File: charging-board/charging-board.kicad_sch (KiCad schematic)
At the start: 53 parts, among them J1 Conn_02x13_Counter_Clockwise, J12 everything_connector, J13 FTSH-107-01-F-DV-K-P-TR, J2 Conn_01x04, J6 TSMP_to_HV, J7 TSMP_to_Banana Jacks, J8 J1772_Negotiation, SW1 Y97KT23B5NAFP, U1 AP63205WU, U2 ISO1044BD, U3 STM32G441KBTx, U7 MIC5504-3.3YM5, Y2 ECS-240-8-37B-CKY-TR

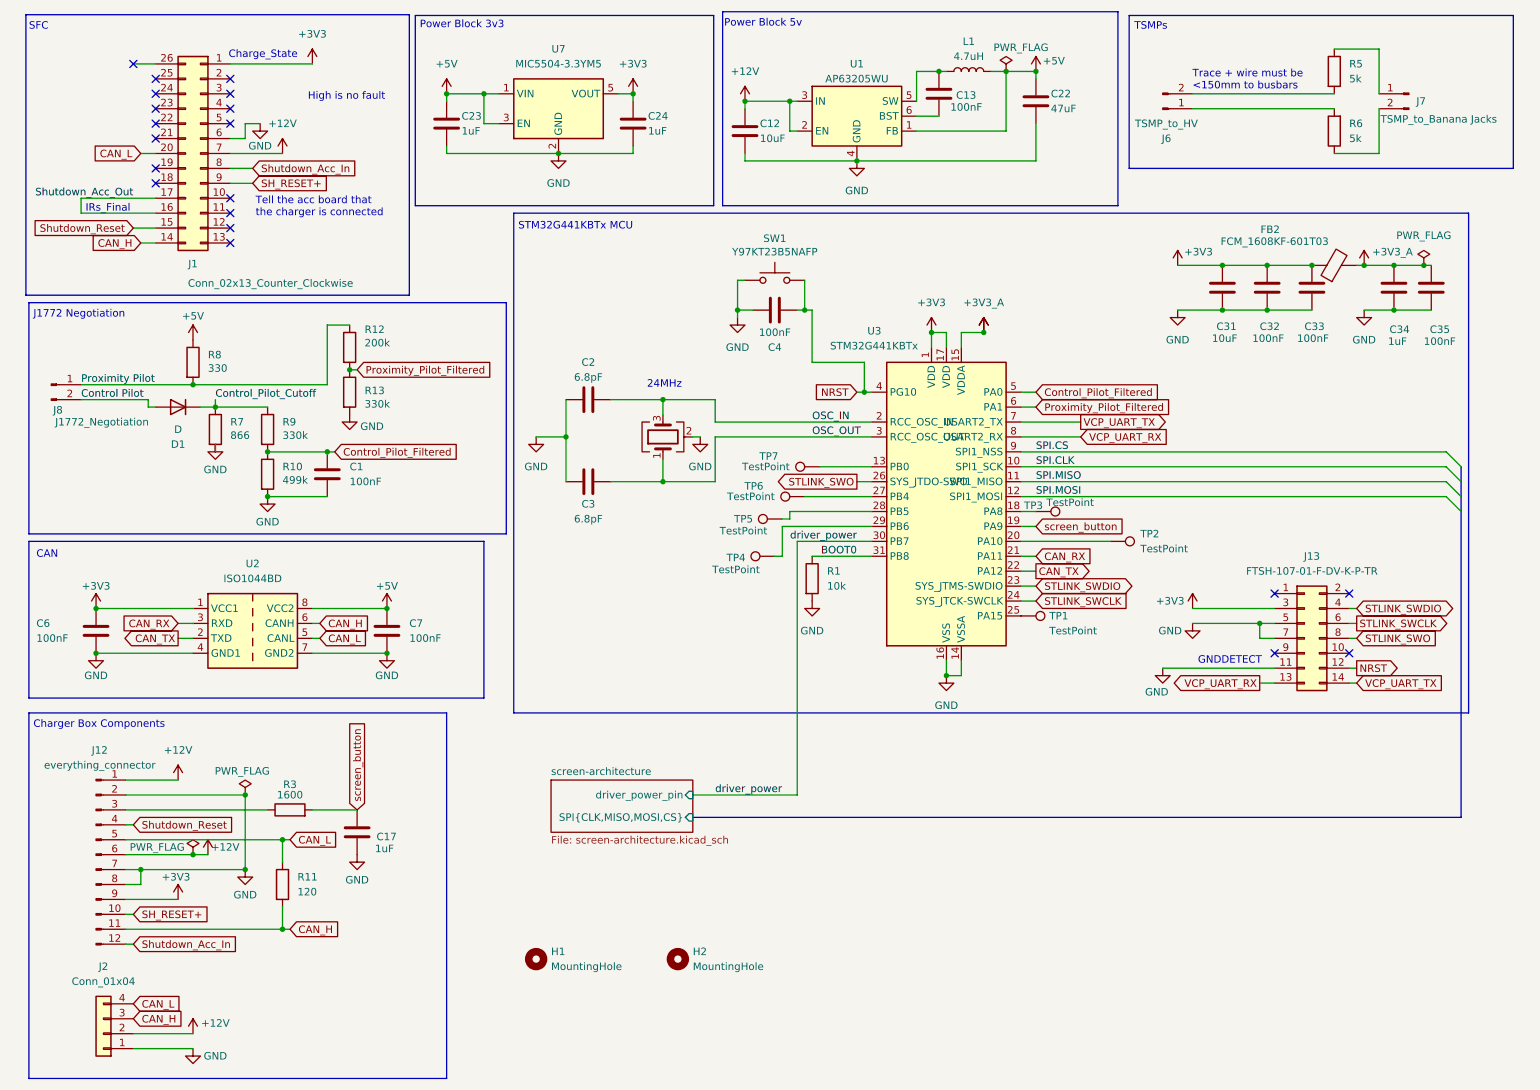
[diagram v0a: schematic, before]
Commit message: added discharge relay
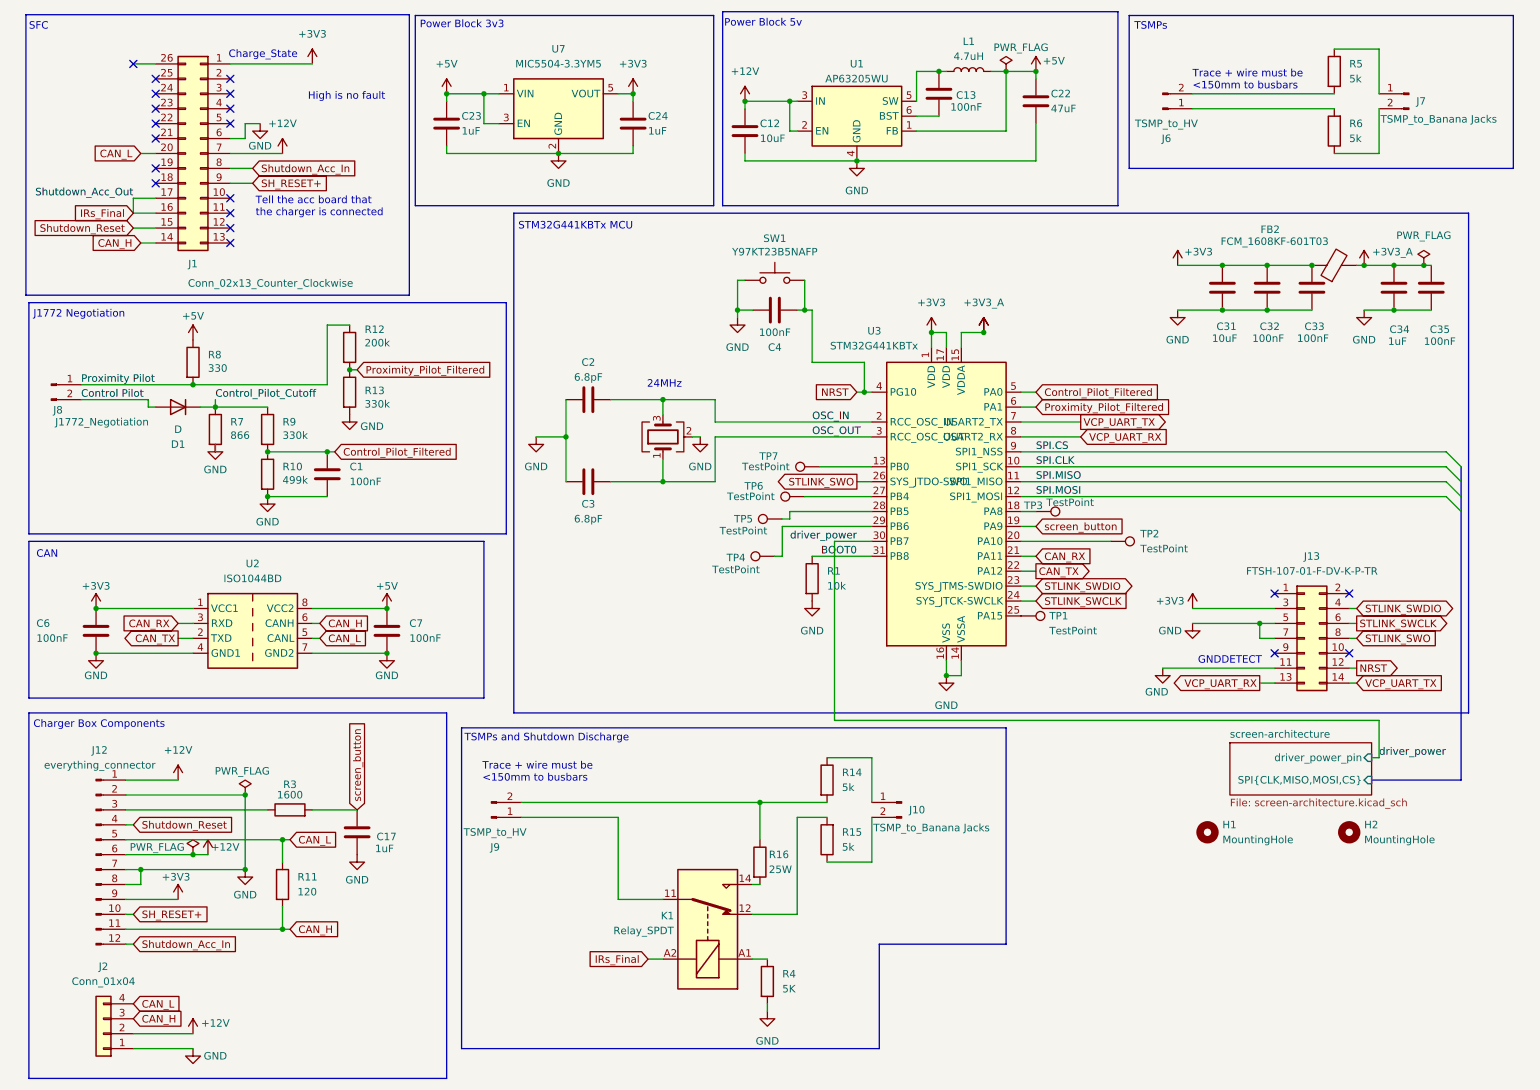
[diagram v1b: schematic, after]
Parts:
- added J10: TSMP_to_Banana Jacks, Connector_Molex:Molex_Nano-Fit_105309-xx02_1x02_P2.50mm_Vertical, symbol Connector:Conn_01x02_Pin
- added J9: TSMP_to_HV, Connector_Molex:Molex_Nano-Fit_105309-xx02_1x02_P2.50mm_Vertical, symbol Connector:Conn_01x02_Pin
- added K1: Relay_SPDT, symbol Relay:Relay_SPDT
- added R14, R15: 5k, Resistor_THT:R_Axial_DIN0922_L20.0mm_D9.0mm_P25.40mm_Horizontal, symbol Device:R
- added R16: 25W, symbol Device:R
- added R4: 5K, symbol Device:R
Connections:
- net GND: now also R4.2
- net Shutdown_Acc_Out renamed IRs_Final
- net IRs_Final: now also K1.A2
- new net: J10.2 (Pin_2), R15.1
- new net: K1.12, R15.2
- new net: J9.1 (Pin_1), K1.11
- new net: J9.2 (Pin_2), R14.2, R16.1
- new net: K1.14, R16.2
- new net: J10.1 (Pin_1), R14.1
- new net: K1.A1, R4.1
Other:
- note added: "TSMPs and Shutdown Discharge"
- note removed: "IRs_Final"
- moved on the sheet: H1, H2
